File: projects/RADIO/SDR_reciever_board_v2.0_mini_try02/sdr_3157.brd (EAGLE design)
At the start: 68 x 75 mm, 69 parts, among them IC1 LM1117-33, IC2 L7805CV, U1 NE5532D, U2 SN74LVC1G3157DBVR, U3 SN74LVC1G3157DBVR

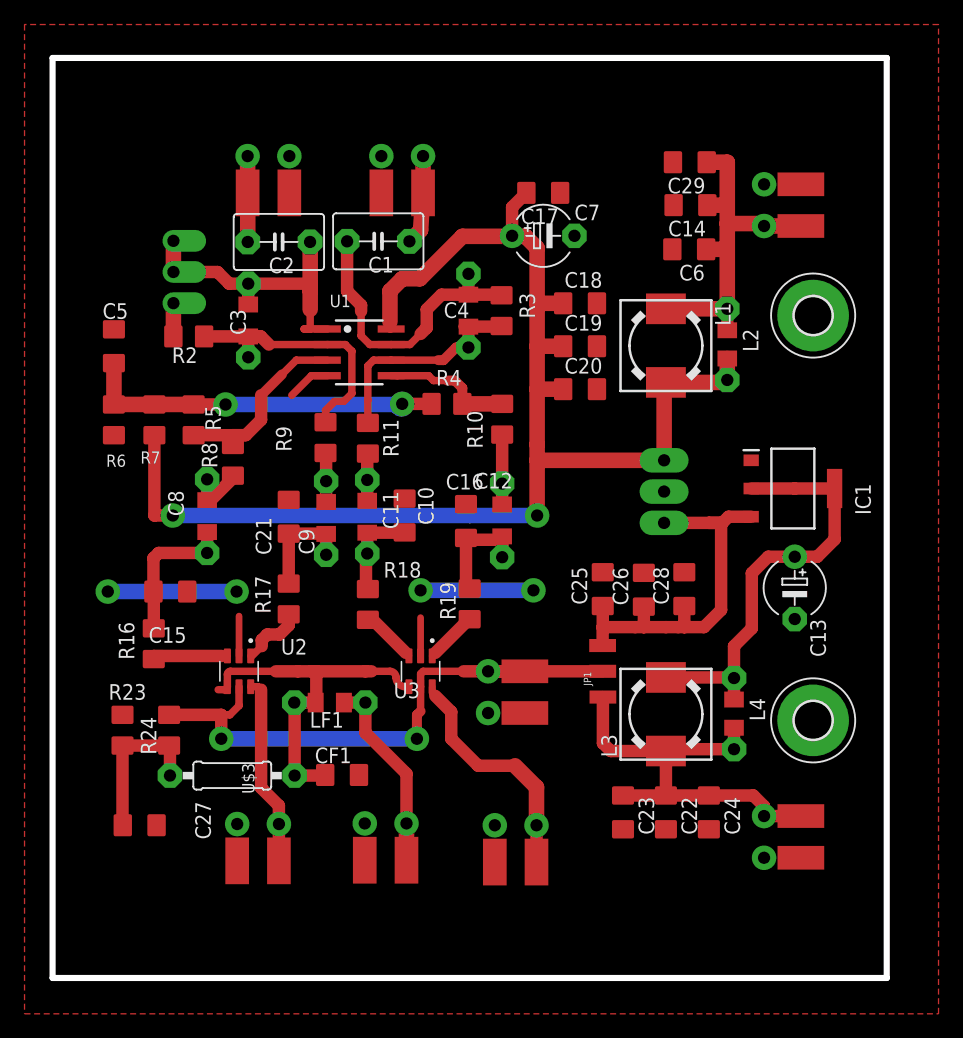
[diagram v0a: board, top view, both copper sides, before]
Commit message: update
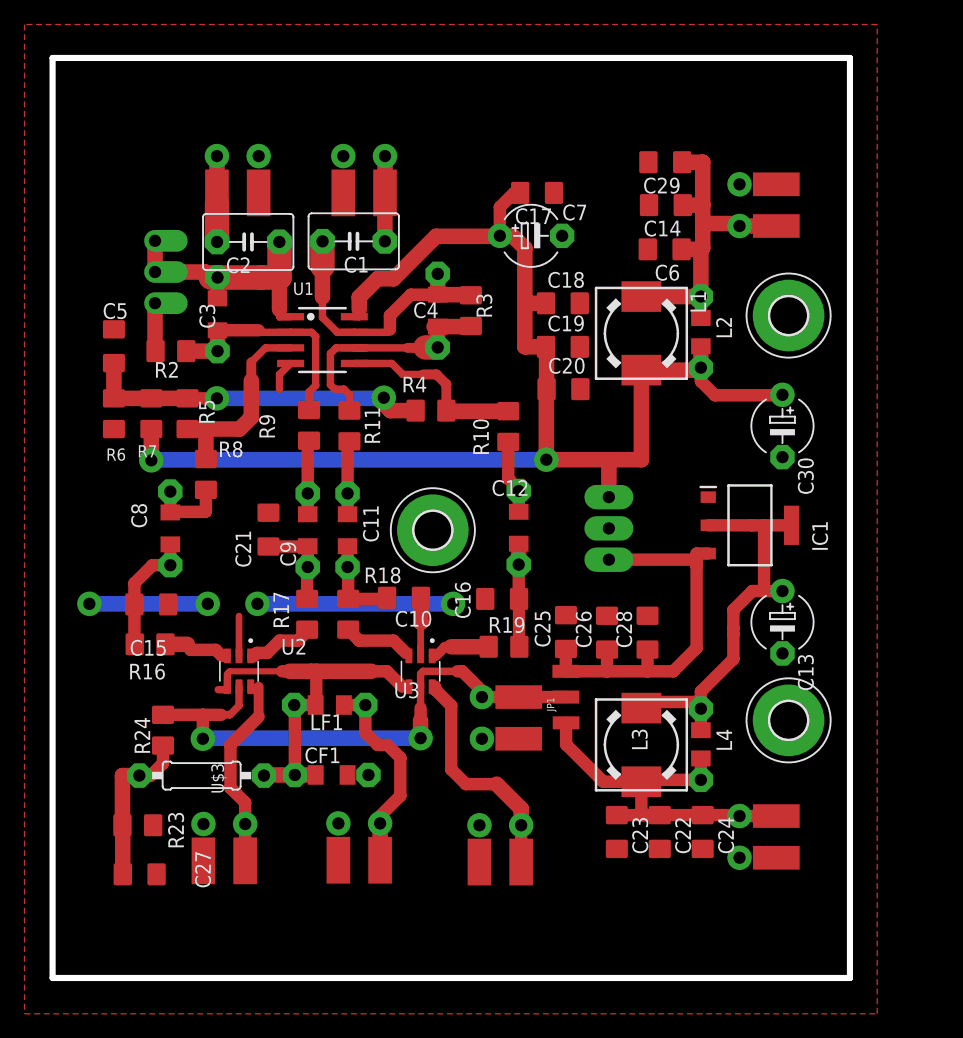
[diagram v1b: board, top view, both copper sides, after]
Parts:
- added C30: (no value), mylib:E5-5
- added H1: MOUNT-PAD-ROUND3.0, holes:3,0-PAD
- CF1: value 22nF -> 150pF; device mylib:C0805 -> mylib:C0805K
- LF1: value 20 -> 390nH
- moved R23 7.85 mm to (6.95, 12.4), turned to 180 degrees
- moved C16 7.00 mm to (36.6, 30.9), turned to 0 degrees
- moved C10 6.70 mm to (28.6, 31.0), turned to 0 degrees
- moved IC2 5.41 mm to (45.4, 39.2)
- moved C28 4.65 mm to (48.5, 28.1)
- moved C25 4.61 mm to (41.9, 28.2)
- moved C26 4.61 mm to (45.2, 28.1)
- moved IC1 4.61 mm to (56.9, 36.9)
- moved R19 4.48 mm to (36.8, 27.0), turned to 0 degrees
- moved C27 4.00 mm to (7.10, 8.45)
- moved L4 3.68 mm to (52.9, 19.1)
- moved JP1 3.66 mm to (42.0, 22.3)
- moved L3 3.20 mm to (48.0, 19.0)
- moved C8 3.16 mm to (9.60, 36.6)
- moved U1 3.16 mm to (22.0, 52.0)
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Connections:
- net 12V: now also C30.+
- net ANTENNA: now also CF1.P$2
- net GND: now also C30.-, CF1.P$1, H1.B3,0
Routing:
- net GND: track 29.6 -> 36.5 mm
- net N$18: track 10.8 -> 15.4 mm
- net N$21: track 25.3 -> 21.6 mm
- net 3.3V: track 35.8 -> 33.0 mm
- net N$17: track 21.4 -> 18.7 mm
- net VCC: track 48.8 -> 46.1 mm
- net N$6: track 35.3 -> 33.0 mm
- net N$14: track 3.87 -> 6.01 mm
- net N$19: track 18.5 -> 20.6 mm
- net N$13: track 4.02 -> 6.04 mm
- net N$11: track 10.4 -> 8.42 mm
- net N$8: track 12.0 -> 10.2 mm
- net N$24: track 24.2 -> 22.5 mm
- net ANTENNA: track 30.5 -> 32.2 mm
- net N$12: track 4.74 -> 6.39 mm
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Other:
- board size 68 x 75 mm -> 65 x 75 mm
